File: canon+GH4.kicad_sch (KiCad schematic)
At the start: 16 parts, among them Q1 2SC1815, Q2 2SC1815, Q3 2SC1815

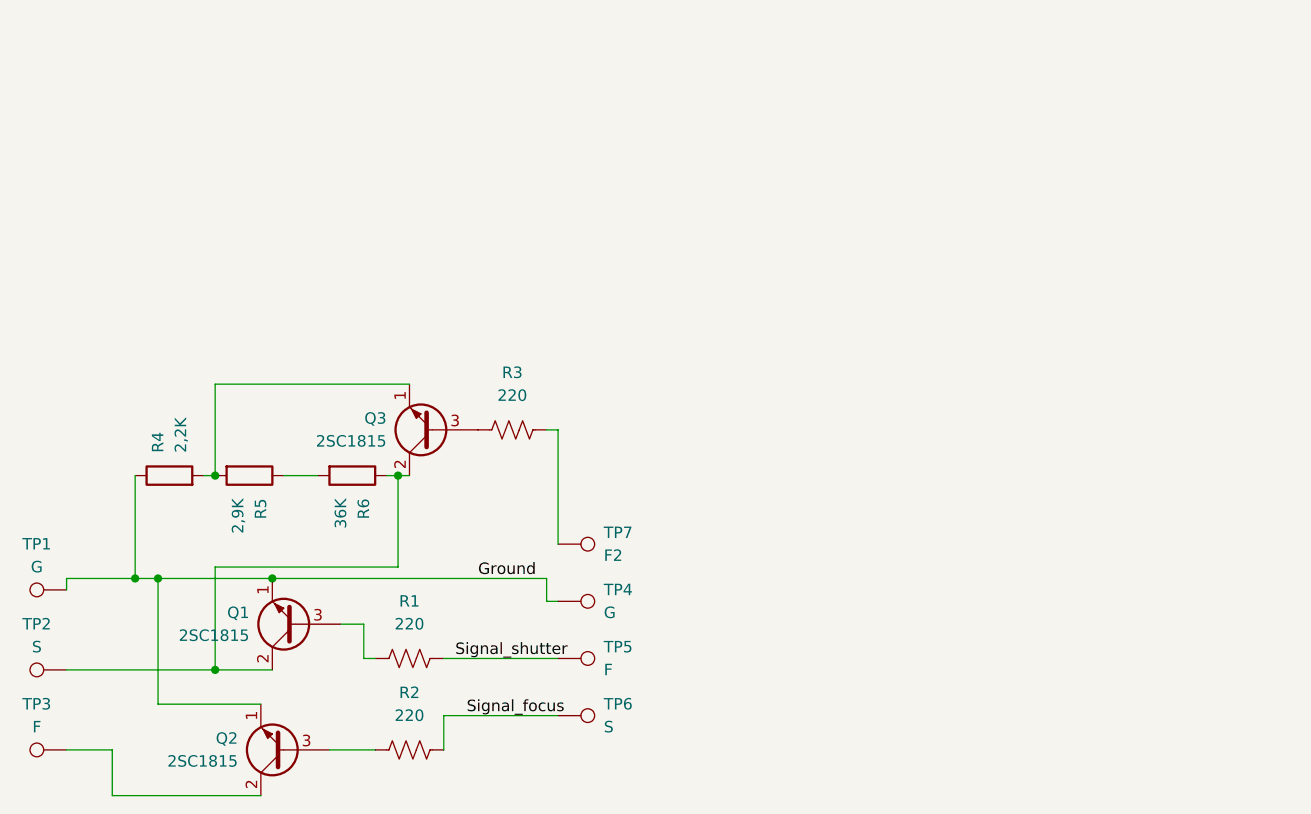
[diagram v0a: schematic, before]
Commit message: updates
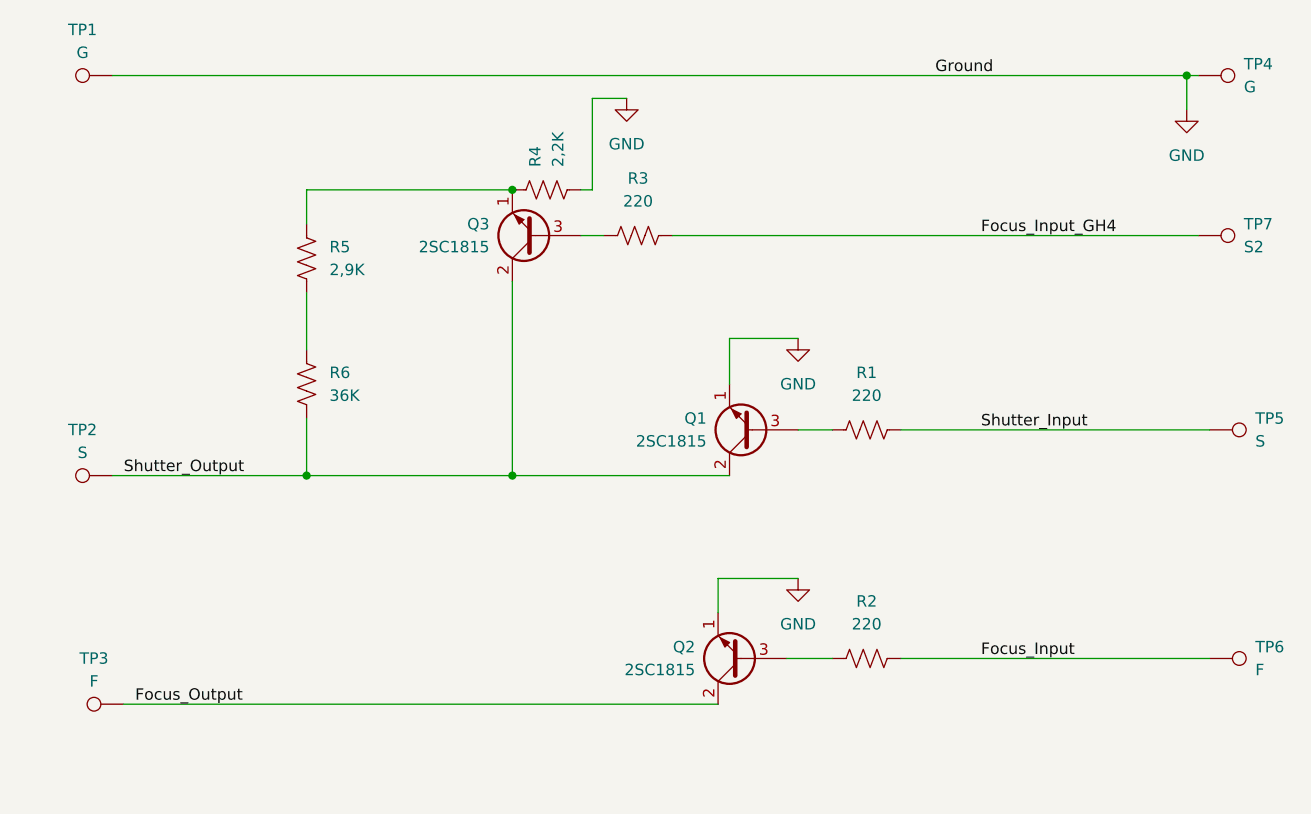
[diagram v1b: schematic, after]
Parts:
- R4, R5, R6: symbol Device:R -> Device:R_US
- TP5: value F -> S
- TP6: value S -> F
- TP7: value F2 -> S2
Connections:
- net Focus_Input_GH4: now reaches R3.1, TP7.1
- net Focus_Output: now reaches Q2.2 (C), TP3.1
- net Shutter_Output: now reaches Q1.2 (C), Q3.2 (C), TP2.1
- net Shutter_Output: now also R6.2; no longer R6.1
- net at R5.1: now also Q3.1 (E), R4.1; no longer R6.2
- net Ground renamed GND
- net GND: now also R4.2; no longer R4.1
- net Signal_focus renamed Focus_Input
- net Signal_shutter renamed Shutter_Input
- new net: R5.2, R6.1
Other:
- moved on the sheet: Q1, Q2, Q3, R1, R2, R3, TP1, TP2, TP3, TP4, TP5, TP6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
